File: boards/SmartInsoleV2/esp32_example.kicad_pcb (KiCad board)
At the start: 2 copper layers, 64.5 x 43.7 mm, 53 parts, among them J1 Conn_01x02_Pin, J2 USB_B_Micro, J3 Conn_01x05_Female, J4 Conn_02x10_Odd_Even, J5 Conn_01x02_Pin, J6 PJS008U-3000-0, J7 Conn_ARM_JTAG_SWD_10, J8 Conn_01x02_Pin, J9 Conn_02x02_Odd_Even, Q2 SS8050-G, Q3 SS8050-G, SW1 SW_Push, SW2 SW_Push, U1 MPU-6050, U3 TLV75801PDRV, U7 ESP32-S3-WROOM-1-N16R2

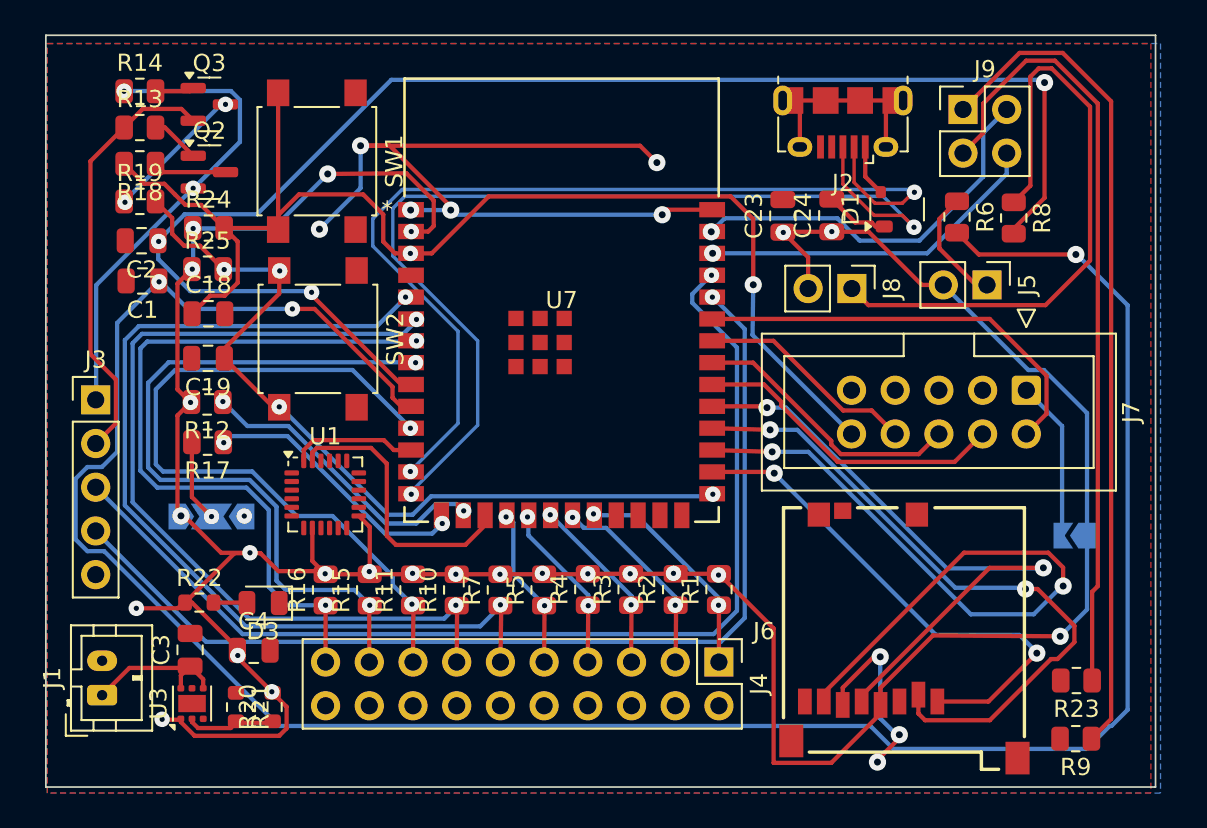
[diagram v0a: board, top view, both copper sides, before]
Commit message: submitted for round 5
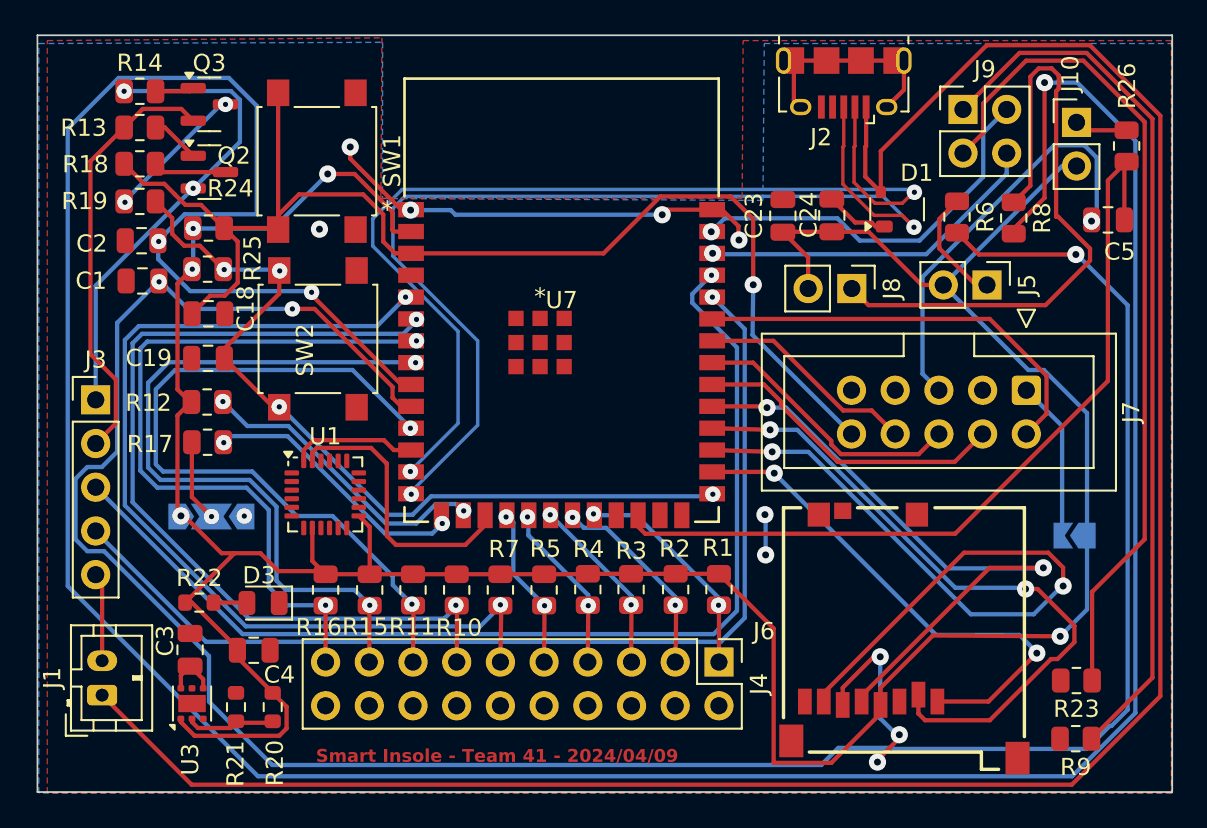
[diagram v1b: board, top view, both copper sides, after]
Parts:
- added C5: 1uF, Capacitor_SMD:C_0805_2012Metric, F.Cu at (225.6, 48.7)
- added J10: Conn_01x02_Pin, Connector_PinHeader_2.54mm:PinHeader_1x02_P2.54mm_Vertical, F.Cu at (223.7, 43.0)
- added R26: 5k, Resistor_SMD:R_0805_2012Metric, F.Cu at (226.6, 44.4)
- moved J2 2.32 mm to (210.2, 40.7)
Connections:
- J1 pad 1: /POWER FROM BATTERY -> +5V
- U7 pad 24: unconnected-(U7-IO47-Pad24) -> /Bluetooth
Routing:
- net +5V: track 3.00 -> 127.7 mm
- net /Start Hike: track 84.3 -> 189.3 mm
- net /Bluetooth: track 0.00 -> 48.4 mm
- net GND: track 63.2 -> 73.1 mm, vias 10 -> 12
- net /POWER FROM BATTERY: track 8.90 -> 3.11 mm
- net Net-(J10-Pin_1): track 0.00 -> 3.78 mm
- net Net-(J9-Pin_3): track 45.8 -> 49.0 mm
- net +3V3: track 174.0 -> 177.0 mm, vias 24 -> 5
- net Net-(J9-Pin_1): track 48.7 -> 51.5 mm
- net /End Hike: track 138.1 -> 140.5 mm
- net /D+: track 59.0 -> 61.3 mm
- net /D-: track 57.1 -> 59.4 mm
- net unconnected-(J2-Shield-Pad6): track 11.5 -> 12.3 mm
- net /RTS: vias 3 -> 2
- net /RX: vias 2 -> 1
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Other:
- board size 64.5 x 43.7 mm -> 65.9 x 44 mm
- board text added: "Smart Insole - Team 41 - 2024/04/09"
